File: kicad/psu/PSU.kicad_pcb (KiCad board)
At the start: 2 copper layers, 54.5 x 54.5 mm, 53 parts, among them J1 B2B-PH-K-S, J2 Conn_01x09_Pin, U1 BQ21040DBVR, U2 RT4812GJ8F, U3 AP3445LW6-7, U4 AP3445LW6-7

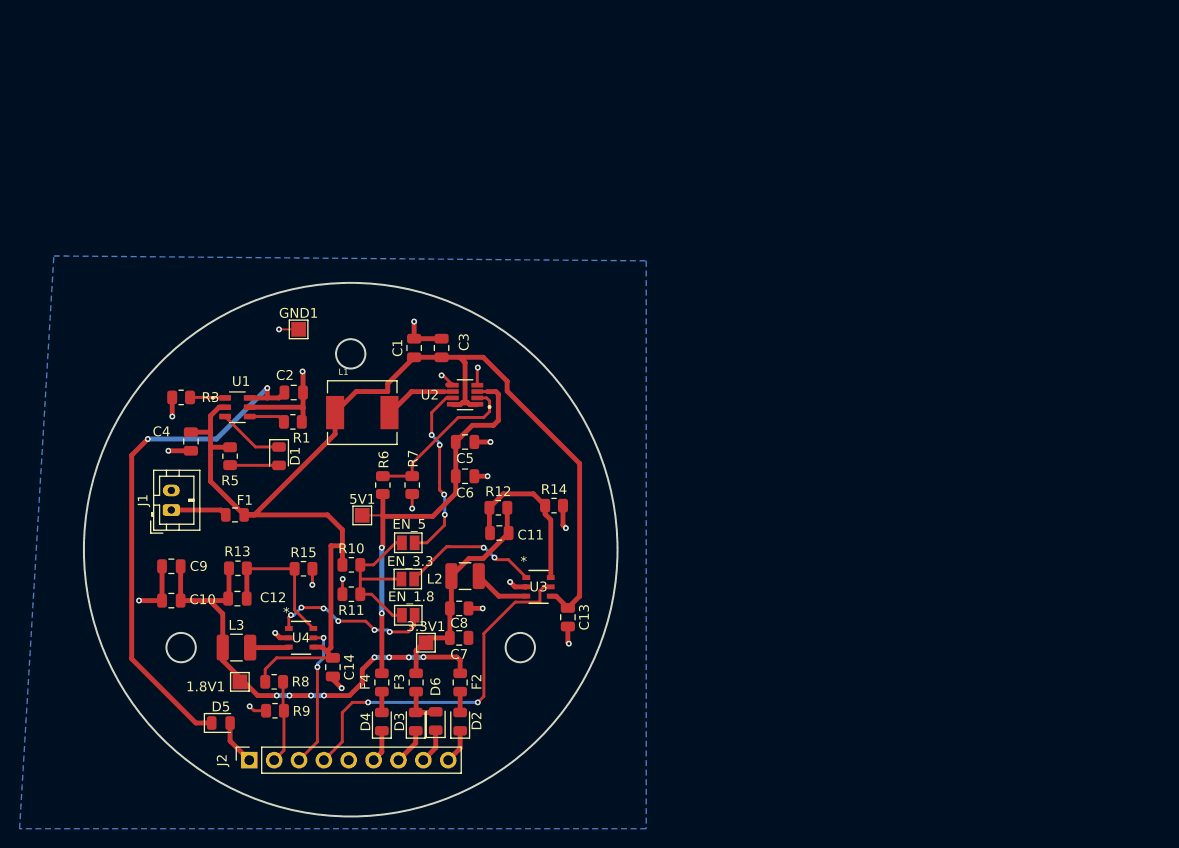
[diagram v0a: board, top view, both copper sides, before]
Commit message: PSU Rev 2
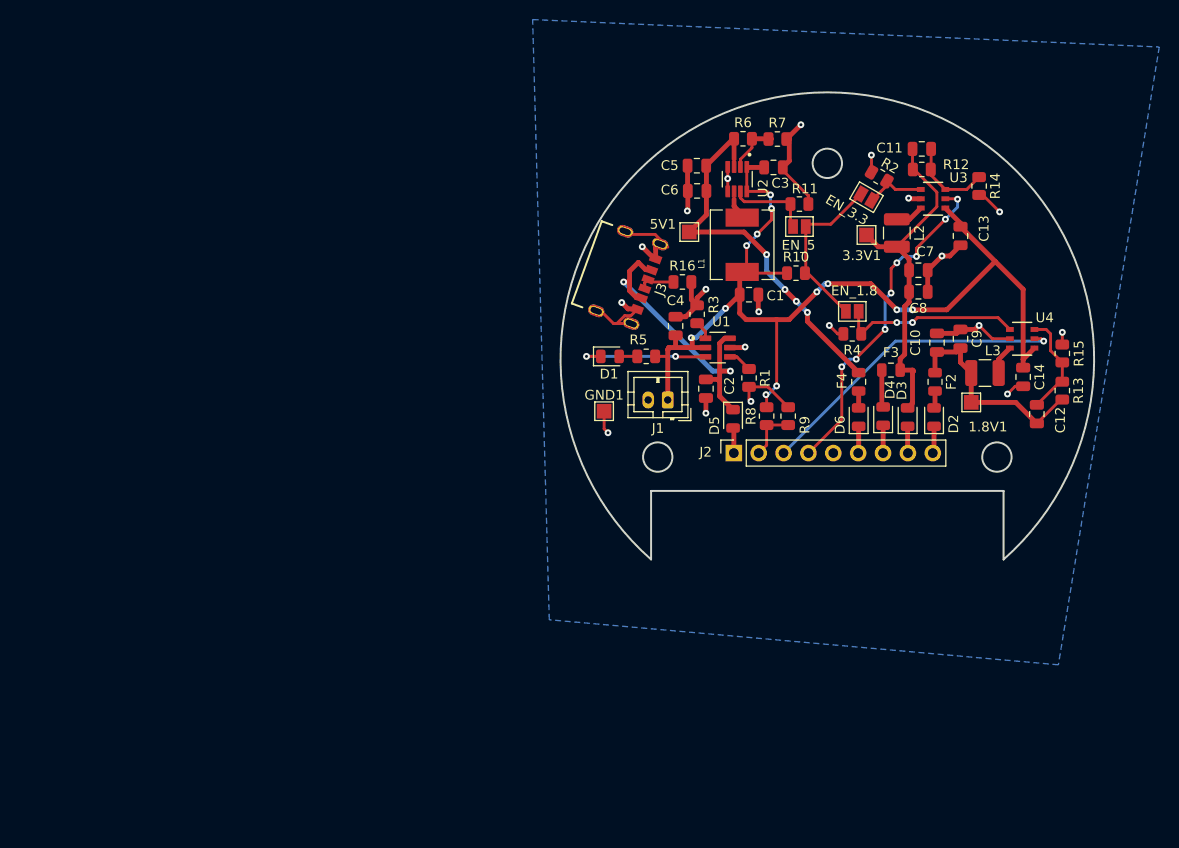
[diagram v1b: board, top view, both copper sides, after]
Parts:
- removed F1: 2A, Fuse:Fuse_0805_2012Metric
- added J3: *, PSAT_Library:GCT_USB4125-GF-A_REVA2, F.Cu at (177.6, 66.3)
- added R16: 22K, Resistor_SMD:R_0805_2012Metric, F.Cu at (184.2, 67.2)
- added R2: 1Meg, Resistor_SMD:R_0805_2012Metric, F.Cu at (204.3, 56.4)
- added R4: 1Meg, Resistor_SMD:R_0805_2012Metric, F.Cu at (201.6, 72.5)
- D2, D3, D4, D5, D6: value D -> D_Schottky
- moved R13 86.1 mm to (223.0, 78.3), turned to -90 degrees
- moved C9 83.9 mm to (212.6, 73.0), turned to -90 degrees
- moved C12 83.8 mm to (220.4, 80.7), turned to 90 degrees
- moved C10 82.5 mm to (210.2, 73.4), turned to -90 degrees
- moved L3 81.4 mm to (215.1, 76.5)
- moved R15 80.6 mm to (223.0, 74.5), turned to 90 degrees
- moved 1.8V1 80.0 mm to (213.7, 79.5), turned to 180 degrees
- moved U4 79.7 mm to (218.9, 73.0)
- moved C14 76.5 mm to (219.0, 76.9)
- moved 3.3V1 61.3 mm to (203.0, 62.4), turned to 180 degrees
- moved EN_3.3 61.0 mm to (203.0, 58.5), turned to 150 degrees
- moved D5 60.8 mm to (189.4, 81.1), turned to -90 degrees
- moved R11 60.7 mm to (196.2, 59.2), turned to 0 degrees
- moved R9 60.4 mm to (195.0, 80.9), turned to 90 degrees
- moved C7 60.1 mm to (208.3, 66.0)
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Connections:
- D3 pad 2: 3.3V -> 3.3V_T
- D4 pad 2: 5V -> 3.3V
- D6 pad 2: 3.3V -> 5V
- J2 pad 6: Net-(D4-K) -> Net-(D6-K)
- J2 pad 7: Net-(D3-K) -> Net-(D4-K)
- J2 pad 8: Net-(D6-K) -> Net-(D3-K)
- R11 pad 1: Net-(EN_1.8-B) -> EN_5
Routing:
- net GND: track 51.6 -> 79.5 mm, vias 20 -> 19
- net 1.8V_T: track 47.9 -> 22.0 mm, vias 8 -> 0
- net Vbat: track 127.8 -> 106.7 mm, vias 0 -> 12
- net Vcharger: track 53.2 -> 32.9 mm
- net PG_1.8: track 14.6 -> 32.4 mm, vias 2 -> 1
- net 3.3V_T: track 23.0 -> 35.4 mm
- net Net-(U2-FB): track 16.9 -> 5.36 mm
- net EN_5: track 18.7 -> 8.34 mm, vias 4 -> 0
- net Net-(U3-FB): track 17.0 -> 8.74 mm
- net EN_3.3: track 14.1 -> 6.41 mm, vias 2 -> 0
- net Net-(D1-K): track 6.80 -> 13.6 mm, vias 0 -> 2
- net 5V_T: track 44.4 -> 38.4 mm, vias 2 -> 4
- net Net-(F1-Pad2): track 5.77 -> 0.00 mm
- net Net-(U2-SW): track 6.55 -> 2.21 mm
- net Net-(U4-FB): track 14.9 -> 10.8 mm
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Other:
- board size 54.5 x 54.5 mm -> 54.5 x 47.7 mm
